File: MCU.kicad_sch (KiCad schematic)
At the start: 12 parts, among them U3 E73-2G4M08S1C, X1 ABS07-LR-32.768KHZ-6-1-T

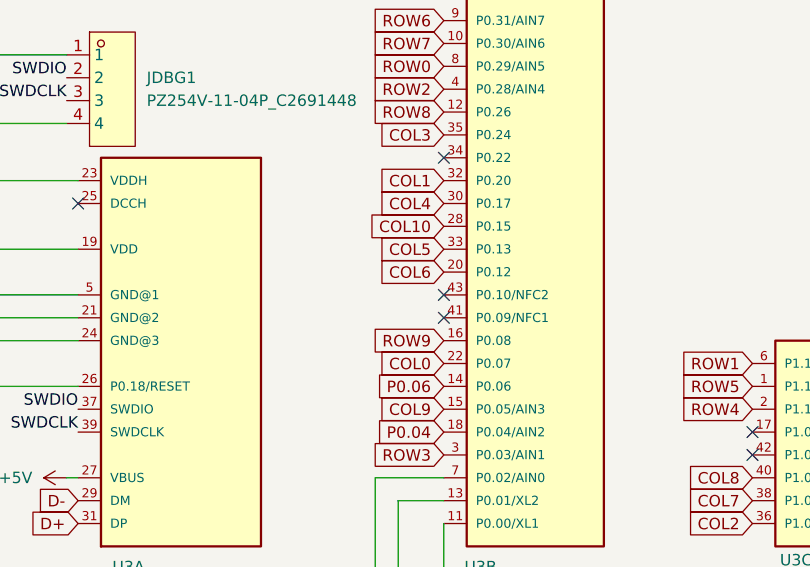
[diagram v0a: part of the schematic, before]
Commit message: v2.3 board ;(
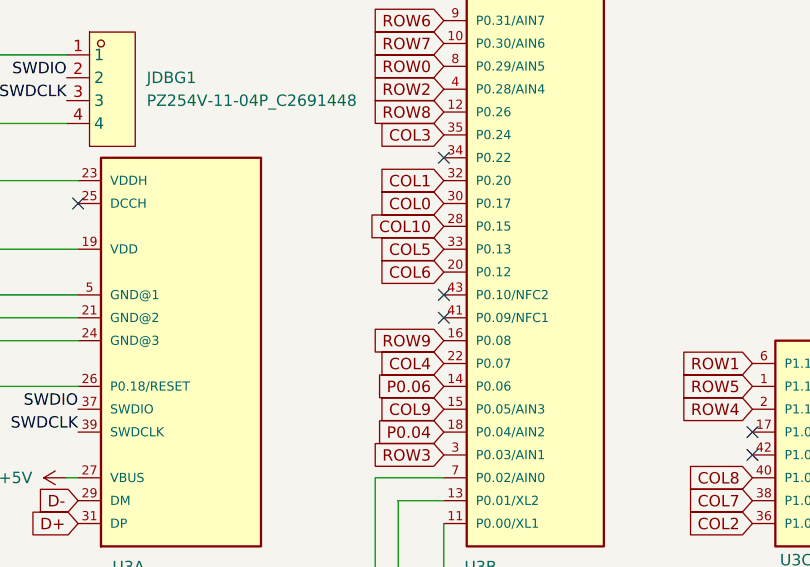
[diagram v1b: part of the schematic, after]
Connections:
- net COL0: now also U3.30 (P0.17); no longer U3.22 (P0.07)
- net COL4: now also U3.22 (P0.07); no longer U3.30 (P0.17)
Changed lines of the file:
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@@
 	(global_label "COL0"
 		(shape input)
-		(at 162.56 80.01 180)
+		(at 162.56 62.23 180)
 		(fields_autoplaced yes)
 		(effects
@@
 		)
 		(property "Intersheetrefs" "${INTERSHEET_REFS}"
-			(at 154.7367 80.01 0)
+			(at 154.7367 62.23 0)
 			(hide yes)
 			(show_name no)
@@
 	(global_label "COL4"
 		(shape input)
-		(at 162.56 62.23 180)
+		(at 162.56 80.01 180)
 		(fields_autoplaced yes)
 		(effects
@@
 		)
 		(property "Intersheetrefs" "${INTERSHEET_REFS}"
-			(at 154.7367 62.23 0)
+			(at 154.7367 80.01 0)
 			(hide yes)
 			(show_name no)
@@
 		)
 		(instances
-			(project "V2"
+			(project "V2.3"
 				(path "/85bcdc0c-8dc1-43cb-ba77-3dcf7ad94591/5a1195dd-ea1d-43d8-8bdb-0580149b420e"
 					(reference "U3")
@@
 		)
 		(instances
-			(project "V2"
+			(project "V2.3"
 				(path "/85bcdc0c-8dc1-43cb-ba77-3dcf7ad94591/5a1195dd-ea1d-43d8-8bdb-0580149b420e"
 					(reference "C10")
@@
 		)
 		(instances
-			(project "V2"
+			(project "V2.3"
 				(path "/85bcdc0c-8dc1-43cb-ba77-3dcf7ad94591/5a1195dd-ea1d-43d8-8bdb-0580149b420e"
 					(reference "RST_S2")
@@
 		)
 		(instances
-			(project "V2"
+			(project "V2.3"
 				(path "/85bcdc0c-8dc1-43cb-ba77-3dcf7ad94591/5a1195dd-ea1d-43d8-8bdb-0580149b420e"
 					(reference "U3")
@@
 		)
 		(instances
-			(project "V2"
+			(project "V2.3"
 				(path "/85bcdc0c-8dc1-43cb-ba77-3dcf7ad94591/5a1195dd-ea1d-43d8-8bdb-0580149b420e"
 					(reference "#PWR04")
@@
 		)
 		(instances
-			(project "V2"
+			(project "V2.3"
 				(path "/85bcdc0c-8dc1-43cb-ba77-3dcf7ad94591/5a1195dd-ea1d-43d8-8bdb-0580149b420e"
 					(reference "#PWR05")
@@
 		)
 		(instances
-			(project "V2"
+			(project "V2.3"
 				(path "/85bcdc0c-8dc1-43cb-ba77-3dcf7ad94591/5a1195dd-ea1d-43d8-8bdb-0580149b420e"
 					(reference "C8")
@@
 		)
 		(instances
-			(project "V2"
+			(project "V2.3"
 				(path "/85bcdc0c-8dc1-43cb-ba77-3dcf7ad94591/5a1195dd-ea1d-43d8-8bdb-0580149b420e"
 					(reference "C5")
@@
 		)
 		(instances
-			(project "V2"
+			(project "V2.3"
 				(path "/85bcdc0c-8dc1-43cb-ba77-3dcf7ad94591/5a1195dd-ea1d-43d8-8bdb-0580149b420e"
 					(reference "C9")
@@
 		)
 		(instances
-			(project "V2"
+			(project "V2.3"
 				(path "/85bcdc0c-8dc1-43cb-ba77-3dcf7ad94591/5a1195dd-ea1d-43d8-8bdb-0580149b420e"
 					(reference "R7")
@@
 		)
 		(instances
-			(project "V2"
+			(project "V2.3"
 				(path "/85bcdc0c-8dc1-43cb-ba77-3dcf7ad94591/5a1195dd-ea1d-43d8-8bdb-0580149b420e"
 					(reference "R6")
@@
 		)
 		(instances
-			(project "V2"
+			(project "V2.3"
 				(path "/85bcdc0c-8dc1-43cb-ba77-3dcf7ad94591/5a1195dd-ea1d-43d8-8bdb-0580149b420e"
 					(reference "#PWR06")
@@
 		)
 		(instances
-			(project "V2"
+			(project "V2.3"
 				(path "/85bcdc0c-8dc1-43cb-ba77-3dcf7ad94591/5a1195dd-ea1d-43d8-8bdb-0580149b420e"
 					(reference "JDBG1")
@@
 		)
 		(instances
-			(project "V2"
+			(project "V2.3"
 				(path "/85bcdc0c-8dc1-43cb-ba77-3dcf7ad94591/5a1195dd-ea1d-43d8-8bdb-0580149b420e"
 					(reference "C7")
@@
 		)
 		(instances
-			(project "V2"
+			(project "V2.3"
 				(path "/85bcdc0c-8dc1-43cb-ba77-3dcf7ad94591/5a1195dd-ea1d-43d8-8bdb-0580149b420e"
 					(reference "X1")
@@
 		)
 		(instances
-			(project "V2"
+			(project "V2.3"
 				(path "/85bcdc0c-8dc1-43cb-ba77-3dcf7ad94591/5a1195dd-ea1d-43d8-8bdb-0580149b420e"
 					(reference "U3")
@@
 		)
 		(instances
-			(project "V2"
+			(project "V2.3"
 				(path "/85bcdc0c-8dc1-43cb-ba77-3dcf7ad94591/5a1195dd-ea1d-43d8-8bdb-0580149b420e"
 					(reference "C6")
